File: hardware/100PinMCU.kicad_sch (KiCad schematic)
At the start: 28 parts, among them J2 SWD_Header_02x02, U3 STM32G491VET6_1, Y1 Crystal

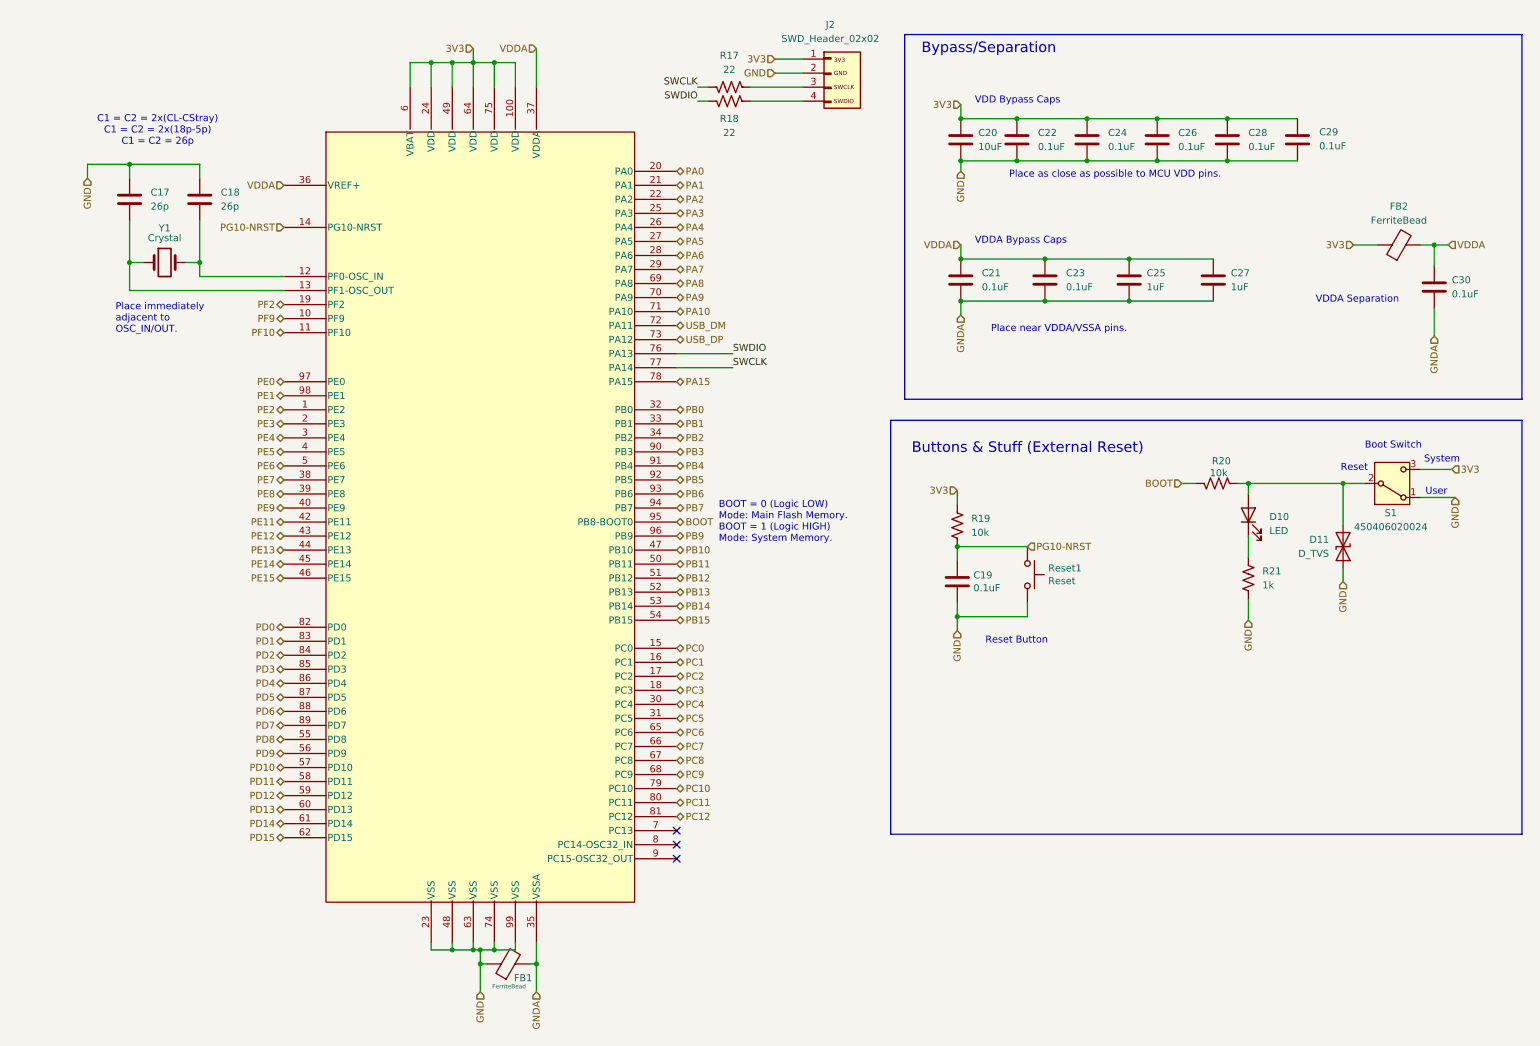
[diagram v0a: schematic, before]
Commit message: added calcs, cleaned up, addressed comments
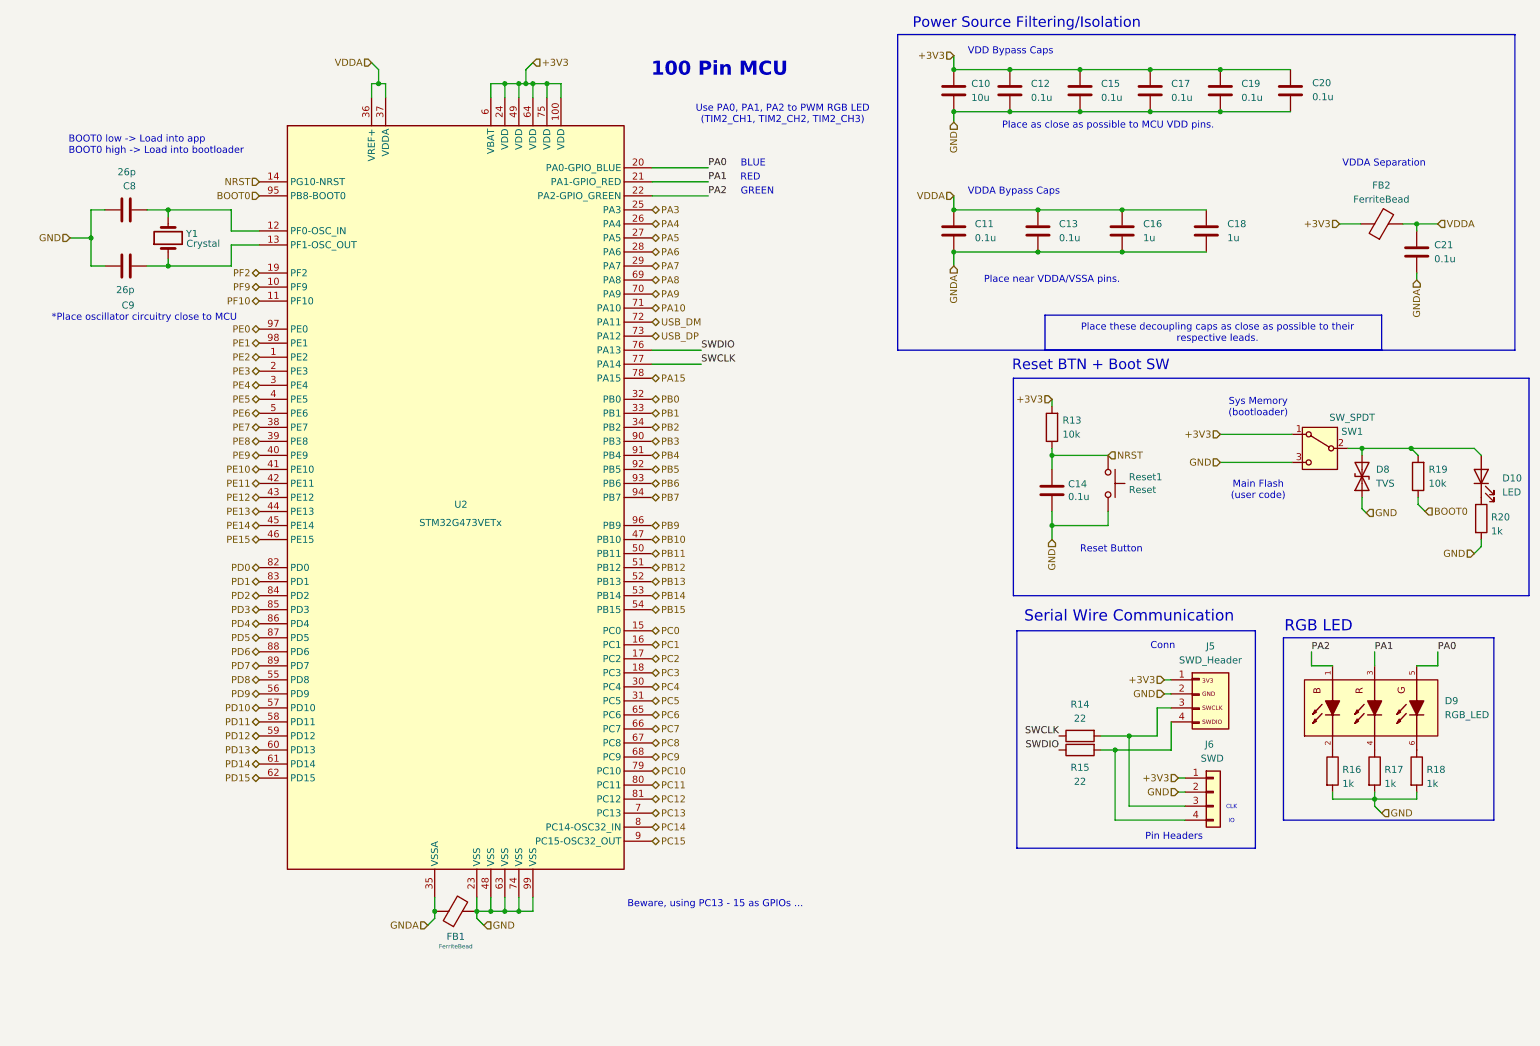
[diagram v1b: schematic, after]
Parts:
- removed C17, C18: 26p, Capacitor_SMD:C_0603_1608Metric_Pad1.08x0.95mm_HandSolder, symbol Device:C
- removed D10: LED, LED_SMD:LED_0201_0603Metric, symbol Device:LED
- removed D11: D_TVS, Diode_SMD:D_SOD-323, symbol Device:D_TVS
- removed R17, R18: 22, Resistor_SMD:R_0603_1608Metric_Pad0.98x0.95mm_HandSolder, symbol Device:R_US
- removed R20: 10k, Resistor_SMD:R_0603_1608Metric_Pad0.98x0.95mm_HandSolder, symbol Device:R_US
- removed R21: 1k, Resistor_SMD:R_0603_1608Metric_Pad0.98x0.95mm_HandSolder, symbol Device:R_US
- removed S1: 450406020024, LHRS_Special:BootSW, symbol Switch:SW_SPDT
- removed U3: STM32G491VET6_1, LHRS_ICs:LQFP_491VET6_STM, symbol lhrs_ics:STM32G491VET6_1
- added C8, C9: 26p, Capacitor_SMD:C_0603_1608Metric_Pad1.08x0.95mm_HandSolder, symbol Device:C
- added D10: LED, LED_SMD:LED_0603_1608Metric, symbol lhrs_misc:Blue_LED
- added D8: TVS, Diode_SMD:D_SOD-323, symbol lhrs_misc:Boot_TVS
- added D9: RGB_LED, LHRS_Special:RGB_LED, symbol lhrs_special:RGB_LED
- added J6: SWD, Connector_PinHeader_2.54mm:PinHeader_1x04_P2.54mm_Vertical, symbol Connector_Generic:Conn_01x04
- added R14, R15: 22, Resistor_SMD:R_0603_1608Metric_Pad0.98x0.95mm_HandSolder, symbol Device:R
- added R16, R17, R18, R20: 1k, Resistor_SMD:R_0603_1608Metric_Pad0.98x0.95mm_HandSolder, symbol Device:R
- added R19: 10k, Resistor_SMD:R_0603_1608Metric_Pad0.98x0.95mm_HandSolder, symbol Device:R
- added SW1: SW_SPDT, LHRS_Special:BootSW, symbol Switch:SW_SPDT
- added U2: STM32G473VETx, LHRS_Special:100PinMCU, symbol lhrs_special:STM32G473VET6
- C10: renamed from C20; value 10uF -> 10u
- C11: renamed from C21; value 0.1uF -> 0.1u
- C12: renamed from C22; value 0.1uF -> 0.1u
- C13: renamed from C23; value 0.1uF -> 0.1u
- C14: renamed from C19; value 0.1uF -> 0.1u
- C15: renamed from C24; value 0.1uF -> 0.1u
- C16: renamed from C25; value 1uF -> 1u
- C17: renamed from C26; value 0.1uF -> 0.1u
- C18: renamed from C27; value 1uF -> 1u
- C19: renamed from C28; value 0.1uF -> 0.1u
- C20: renamed from C29; value 0.1uF -> 0.1u
- C21: renamed from C30; value 0.1uF -> 0.1u
- J5: renamed from J2; value SWD_Header_02x02 -> SWD_Header
- R13: renamed from R19; symbol Device:R_US -> Device:R
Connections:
- net GND: now also FB1.2, C8.1, C9.1, D8.1 (A1), J6.2 (Pin_2), R16.2, R17.2, R18.2, R20.2, SW1.3 (C), U2.23 (VSS), U2.48 (VSS), U2.63 (VSS), U2.74 (VSS), U2.99 (VSS); no longer FB1.1
- net GNDA: now also FB1.1, U2.35 (VSSA); no longer FB1.2
- net PA0: now also D9.5, U2.20 (PA0-GPIO_BLUE)
- net PA1: now also D9.3, U2.21 (PA1-GPIO_RED)
- net PA10: now also U2.71 (PA10)
- net PA15: now also U2.78 (PA15)
- net PA2: now also D9.1, U2.22 (PA2-GPIO_GREEN)
- net PA3: now also U2.25 (PA3)
- net PA4: now also U2.26 (PA4)
- net PA5: now also U2.27 (PA5)
- net PA6: now also U2.28 (PA6)
- net PA7: now also U2.29 (PA7)
- net PA8: now also U2.69 (PA8)
- net PA9: now also U2.70 (PA9)
- net PB0: now also U2.32 (PB0)
- net PB1: now also U2.33 (PB1)
- net PB10: now also U2.47 (PB10)
- net PB11: now also U2.50 (PB11)
- net PB12: now also U2.51 (PB12)
- net PB13: now also U2.52 (PB13)
- net PB14: now also U2.53 (PB14)
- net PB15: now also U2.54 (PB15)
- net PB2: now also U2.34 (PB2)
- net PB3: now also U2.90 (PB3)
- net PB4: now also U2.91 (PB4)
- net PB5: now also U2.92 (PB5)
- net PB6: now also U2.93 (PB6)
- net PB7: now also U2.94 (PB7)
- net PB9: now also U2.96 (PB9)
- net PC0: now also U2.15 (PC0)
- net PC1: now also U2.16 (PC1)
- net PC10: now also U2.79 (PC10)
- net PC11: now also U2.80 (PC11)
- net PC12: now also U2.81 (PC12)
- net PC2: now also U2.17 (PC2)
- net PC3: now also U2.18 (PC3)
- net PC4: now also U2.30 (PC4)
- net PC5: now also U2.31 (PC5)
- net PC6: now also U2.65 (PC6)
- net PC7: now also U2.66 (PC7)
- net PC8: now also U2.67 (PC8)
- net PC9: now also U2.68 (PC9)
- net PD0: now also U2.82 (PD0)
- net PD1: now also U2.83 (PD1)
- net PD10: now also U2.57 (PD10)
- net PD11: now also U2.58 (PD11)
- net PD12: now also U2.59 (PD12)
- net PD13: now also U2.60 (PD13)
- net PD14: now also U2.61 (PD14)
- net PD15: now also U2.62 (PD15)
- net PD2: now also U2.84 (PD2)
- net PD3: now also U2.85 (PD3)
- net PD4: now also U2.86 (PD4)
- net PD5: now also U2.87 (PD5)
- net PD6: now also U2.88 (PD6)
- net PD7: now also U2.89 (PD7)
- net PD8: now also U2.55 (PD8)
- net PD9: now also U2.56 (PD9)
- net PE0: now also U2.97 (PE0)
- net PE1: now also U2.98 (PE1)
- net PE11: now also U2.42 (PE11)
- net PE12: now also U2.43 (PE12)
- net PE13: now also U2.44 (PE13)
- net PE14: now also U2.45 (PE14)
- net PE15: now also U2.46 (PE15)
- net PE2: now also U2.1 (PE2)
- net PE3: now also U2.2 (PE3)
- net PE4: now also U2.3 (PE4)
- net PE5: now also U2.4 (PE5)
- net PE6: now also U2.5 (PE6)
- net PE7: now also U2.38 (PE7)
- net PE8: now also U2.39 (PE8)
- net PE9: now also U2.40 (PE9)
- net PF10: now also U2.11 (PF10)
- net PF2: now also U2.19 (PF2)
- net PF9: now also U2.10 (PF9)
- net SWCLK: now also R14.1, U2.77 (PA14)
- net SWDIO: now also R15.1, U2.76 (PA13)
- net USB_DM: now also U2.72 (PA11)
- net USB_DP: now also U2.73 (PA12)
- net VDDA: now also U2.36 (VREF+), U2.37 (VDDA)
- net at Y1.1: now also C9.2, U2.13 (PF1-OSC_OUT)
- net at Y1.2: now also C8.2, U2.12 (PF0-OSC_IN)
- net at J5.3 (Pin_3): now also J6.3 (Pin_3), R14.2
- net at J5.4 (Pin_4): now also J6.4 (Pin_4), R15.2
- net 3V3 renamed +3V3
- net +3V3: now also J6.1 (Pin_1), SW1.1 (A), U2.100 (VDD), U2.24 (VDD), U2.49 (VDD), U2.6 (VBAT), U2.64 (VDD), U2.75 (VDD)
- net PG10-NRST renamed NRST
- net NRST: now also U2.14 (PG10-NRST)
- new net: D10.1 (K), R20.1
- new net: D10.2 (A), D8.2 (A2), R19.2, SW1.2 (B)
- new net: D9.2, R16.1
- new net: D9.4, R17.1
- new net: D9.6, R18.1
- new net BOOT0: R19.1, U2.95 (PB8-BOOT0)
- new net PC13: U2.7 (PC13)
- new net PC14: U2.8 (PC14-OSC32_IN)
- new net PC15: U2.9 (PC15-OSC32_OUT)
- new net PE10: U2.41 (PE10)
- no-connect marks 3 -> 0
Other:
- note added: "*Place oscillator circuitry close to MCU"
- note added: "100 Pin MCU"
- note added: "BLUE"
- note added: "BOOT0 low -> Load into app BOOT0 high -> Load into bootloader"
- note added: "Beware, using PC13 - 15 as GPIOs ..."
- note added: "CLK"
- note added: "Conn"
- note added: "GREEN"
- note added: "IO"
- note added: "Main Flash (user code)"
- note added: "Pin Headers"
- note added: "Place these decoupling caps as close as possible to their respective leads."
- note added: "Power Source Filtering/Isolation"
- note added: "RED"
- note added: "RGB LED"
- note added: "Reset BTN + Boot SW"
- note added: "Serial Wire Communication"
- note added: "Sys Memory (bootloader)"
- note added: "Use PA0, PA1, PA2 to PWM RGB LED (TIM2_CH1, TIM2_CH2, TIM2_CH3)"
- note removed: "BOOT = 0 (Logic LOW) Mode: Main Flash Memory. BOOT = 1 (Logic HIGH) Mode: System Memory."
- note removed: "Boot Switch"
- note removed: "Buttons & Stuff (External Reset)"
- note removed: "Bypass/Separation"
- note removed: "C1 = C2 = 2x(CL-CStray) C1 = C2 = 2x(18p-5p) C1 = C2 = 26p"
- note removed: "Place immediately adjacent to OSC_IN/OUT."
- note removed: "Reset"
- note removed: "System"
- note removed: "User"
- moved on the sheet: C10, C11, C12, C13, C14, C15, C16, C17, C18, C19, C20, C21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
